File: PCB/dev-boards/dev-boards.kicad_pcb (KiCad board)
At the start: 2 copper layers, 133 x 180 mm, 7 parts, among them J1 5V Input, J2 SIM7600 Cell Header, U1 NUCLEO-F429ZI, U2 NUCLEO-F429ZI

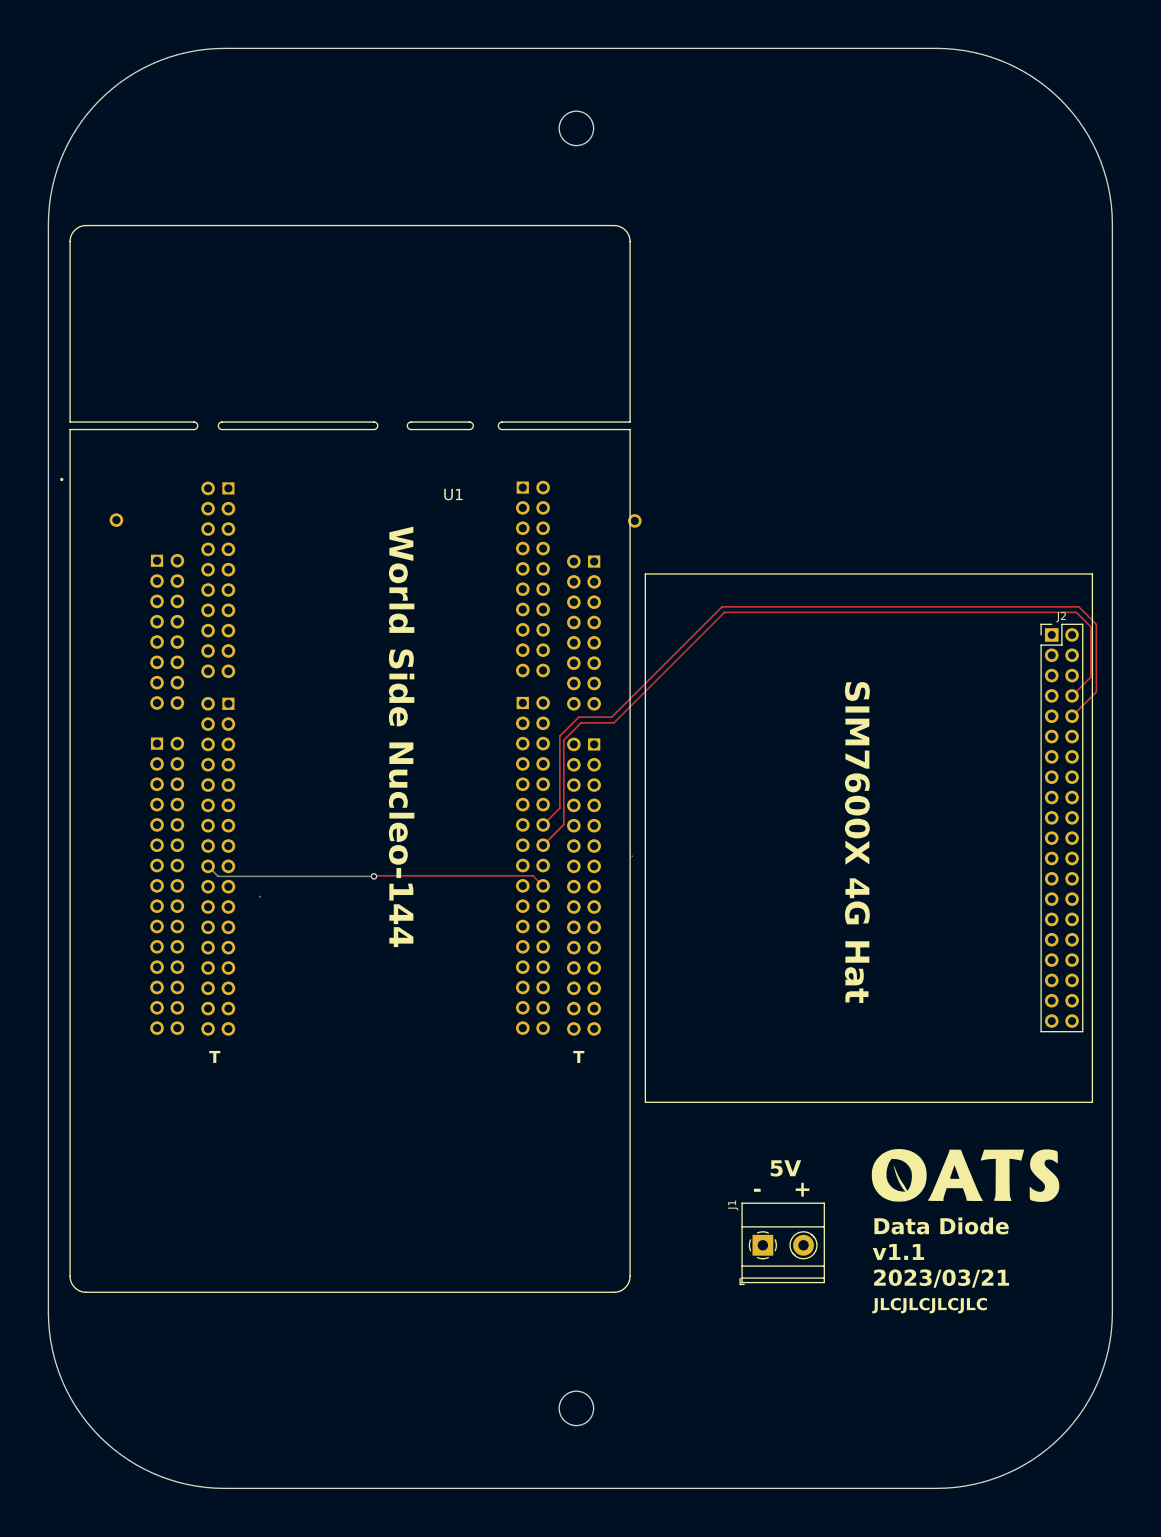
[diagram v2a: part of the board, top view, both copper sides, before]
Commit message: PCB: Edits for 3d box
Signed-off-by: Andrew Balmos <abalmos@purdue.edu>
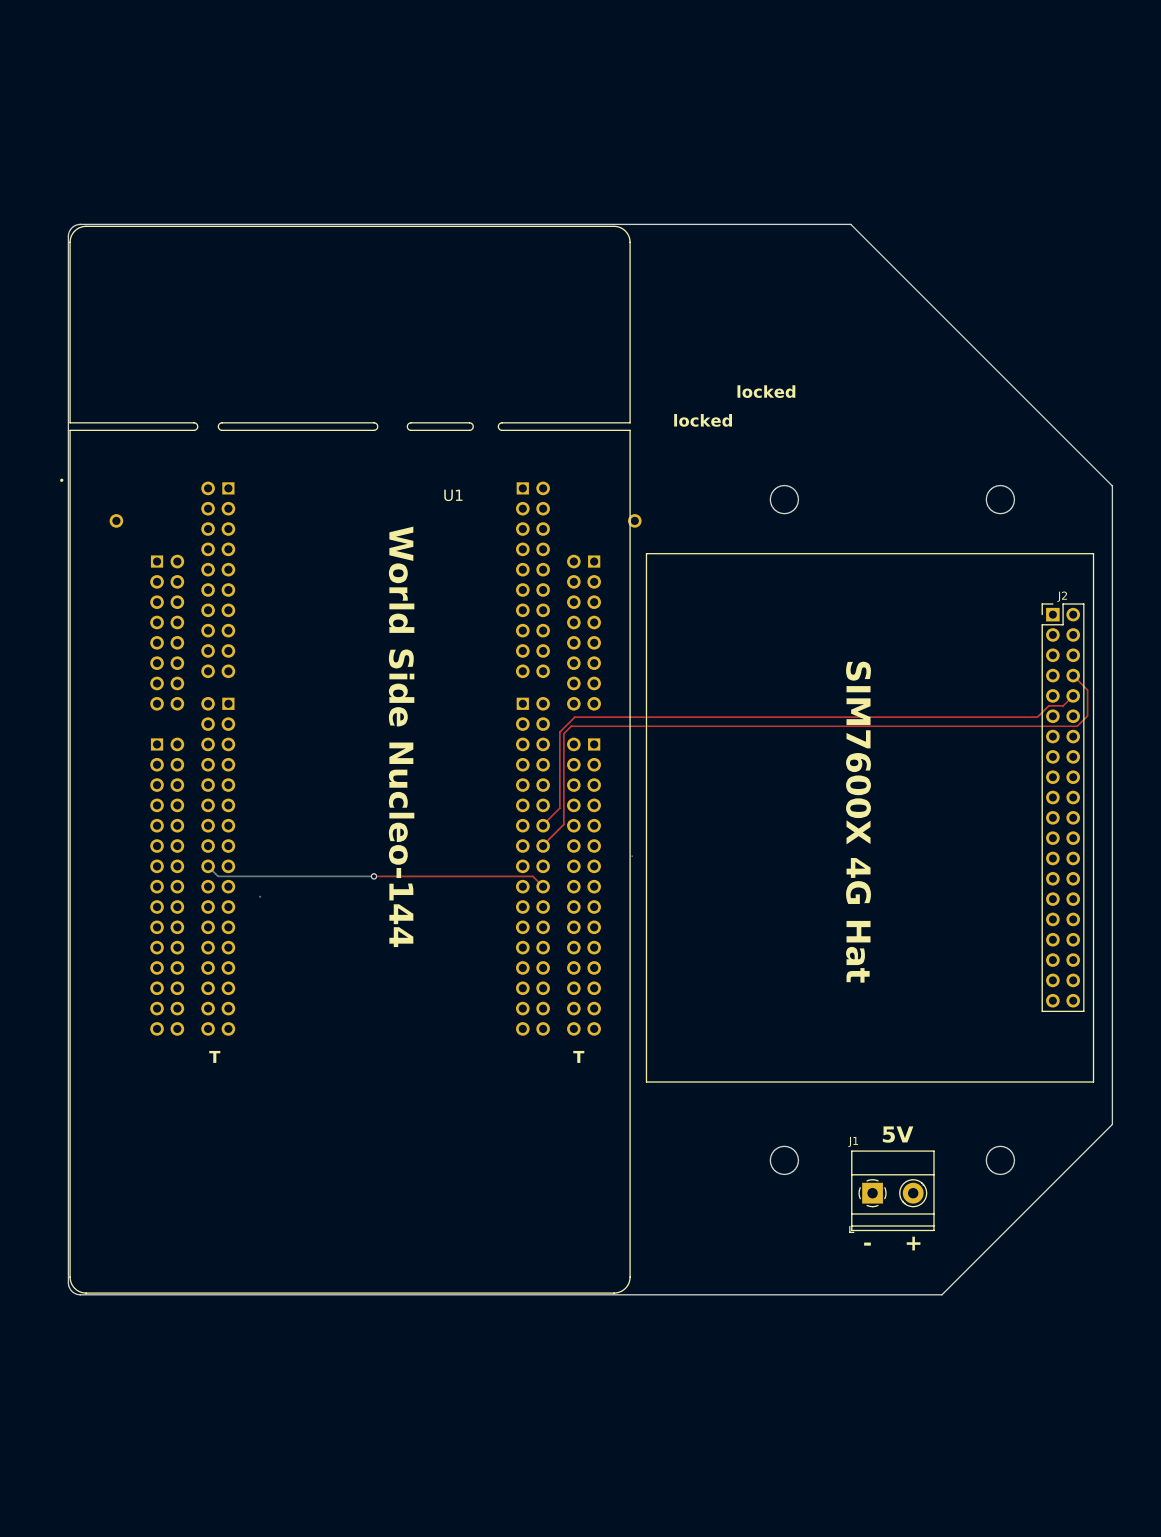
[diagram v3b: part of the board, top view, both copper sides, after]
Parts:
- added G***: LOGO, Local footprints:ccat_logo, F.Cu at (102.4, 47.4)
- added H3: MountingHole, MountingHole:MountingHole_3.5mm, F.Cu at (113.5, 154.5)
- added H4: MountingHole, MountingHole:MountingHole_3.5mm, F.Cu at (140.5, 154.5)
- H1, H2: footprint MountingHole:MountingHole_4.3mm_M4 -> MountingHole:MountingHole_3.5mm
- moved H2 125.4 mm to (140.5, 71.9)
- moved N1 111.0 mm to (118.5, 47.1)
- moved H1 53.2 mm to (113.5, 71.9)
- moved J1 15.2 mm to (124.5, 158.6)
- moved J2 2.54 mm to (147.1, 86.3)
- moved U1 0.10 mm to (59.2, 104.4)
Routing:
- net /M_RX_TX: track 99.4 -> 78.5 mm
- net /M_TX_RX: track 97.1 -> 87.2 mm
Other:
- board size 133 x 180 mm -> 130.5 x 133.8 mm
- board text added: "locked"
- board text removed: "Data Diode v1.1 2023/03/21"
- board text removed: "JLCJLCJLCJLC"
